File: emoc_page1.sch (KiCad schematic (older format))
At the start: 25 parts, among them U2 DRV8323R

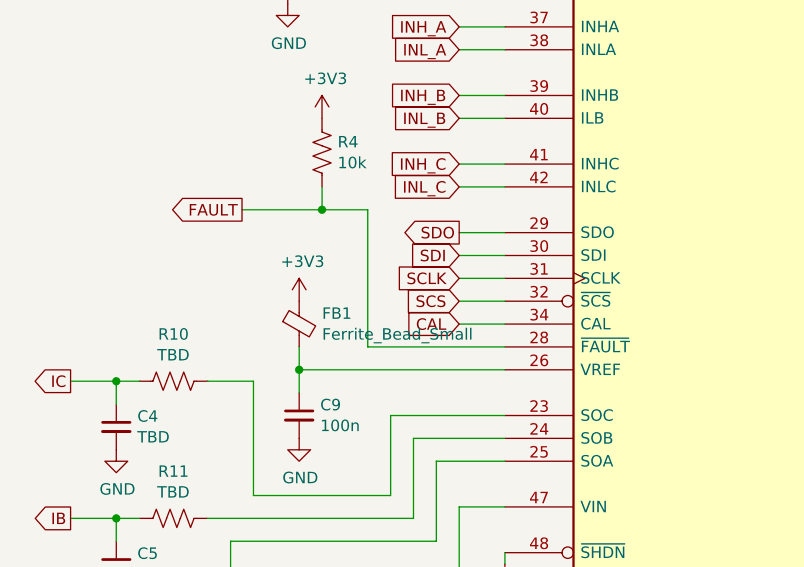
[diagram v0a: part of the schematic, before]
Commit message: still work in progress
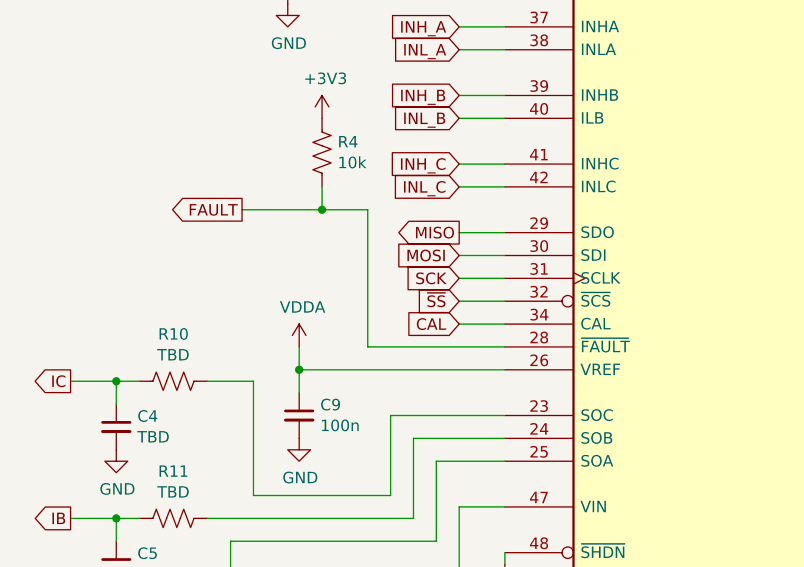
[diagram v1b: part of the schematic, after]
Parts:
- removed FB1: Ferrite_Bead_Small, symbol Device:Ferrite_Bead_Small
- C4, C5, C6, C9: footprint (none) -> Capacitor_SMD:C_0603_1608Metric
- NT1: footprint (none) -> NetTie:NetTie-2_SMD_Pad0.5mm
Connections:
- net VDDA: now reaches C9.1, U2.26 (VREF)
- net SCLK renamed SCK
- net SCS renamed ~SS
- net SDI renamed MOSI
- net SDO renamed MISO
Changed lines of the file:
@@
 $Descr A4 11693 8268
 encoding utf-8
-Sheet 2 4
+Sheet 2 5
 Title ""
 Date ""
@@
 F 0 "NT1" H 5950 1731 50  0000 C CNN
 F 1 "Net-Tie_2" H 5950 1640 50  0000 C CNN
-F 2 "" H 5950 1550 50  0001 C CNN
+F 2 "NetTie:NetTie-2_SMD_Pad0.5mm" H 5950 1550 50  0001 C CNN
 F 3 "~" H 5950 1550 50  0001 C CNN
 	1    5950 1550
@@
 $EndComp
 Text GLabel 3250 3650 0    50   Output ~ 0
-SDO
+MISO
 Text GLabel 3250 3750 0    50   Input ~ 0
-SDI
+MOSI
 Text GLabel 3250 3850 0    50   Input ~ 0
-SCLK
+SCK
 Text GLabel 3250 3950 0    50   Input ~ 0
-SCS
+~SS
 Wire Wire Line
 	3250 3750 3450 3750
@@
 F 0 "C9" H 2642 4496 50  0000 L CNN
 F 1 "100n" H 2642 4405 50  0000 L CNN
-F 2 "" H 2550 4450 50  0001 C CNN
+F 2 "Capacitor_SMD:C_0603_1608Metric" H 2550 4450 50  0001 C CNN
 F 3 "~" H 2550 4450 50  0001 C CNN
 	1    2550 4450
@@
 	2550 4250 2550 4150
 Connection ~ 2550 4250
-$Comp
-L power:+3V3 #PWR0110
-U 1 1 5FF033F4
-P 2550 3950
-F 0 "#PWR0110" H 2550 3800 50  0001 C CNN
-F 1 "+3V3" H 2565 4123 50  0000 C CNN
-F 2 "" H 2550 3950 50  0001 C CNN
-F 3 "" H 2550 3950 50  0001 C CNN
-	1    2550 3950
-	1    0    0    -1
-$EndComp
-$Comp
-L Device:Ferrite_Bead_Small FB1
-U 1 1 5FF0A0D9
-P 2550 4050
-F 0 "FB1" H 2650 4096 50  0000 L CNN
-F 1 "Ferrite_Bead_Small" H 2650 4005 50  0000 L CNN
-F 2 "" V 2480 4050 50  0001 C CNN
-F 3 "~" H 2550 4050 50  0001 C CNN
-	1    2550 4050
-	1    0    0    -1
-$EndComp
 Text GLabel 1550 5450 0    50   Output ~ 0
 IA
@@
 F 0 "C6" H 1842 5696 50  0000 L CNN
 F 1 "TBD" H 1842 5605 50  0000 L CNN
-F 2 "" H 1750 5650 50  0001 C CNN
+F 2 "Capacitor_SMD:C_0603_1608Metric" H 1750 5650 50  0001 C CNN
 F 3 "~" H 1750 5650 50  0001 C CNN
 	1    1750 5650
@@
 F 0 "C5" H 1842 5146 50  0000 L CNN
 F 1 "TBD" H 1842 5055 50  0000 L CNN
-F 2 "" H 1750 5100 50  0001 C CNN
+F 2 "Capacitor_SMD:C_0603_1608Metric" H 1750 5100 50  0001 C CNN
 F 3 "~" H 1750 5100 50  0001 C CNN
 	1    1750 5100
@@
 F 0 "C4" H 1842 4546 50  0000 L CNN
 F 1 "TBD" H 1842 4455 50  0000 L CNN
-F 2 "" H 1750 4500 50  0001 C CNN
+F 2 "Capacitor_SMD:C_0603_1608Metric" H 1750 4500 50  0001 C CNN
 F 3 "~" H 1750 4500 50  0001 C CNN
 	1    1750 4500
@@
 Wire Wire Line
 	7200 4200 7200 4300
+$Comp
+L power:VDDA #PWR08
+U 1 1 5FF1727A
+P 2550 4150
+F 0 "#PWR08" H 2550 4000 50  0001 C CNN
+F 1 "VDDA" H 2565 4323 50  0000 C CNN
+F 2 "" H 2550 4150 50  0001 C CNN
+F 3 "" H 2550 4150 50  0001 C CNN
+	1    2550 4150
+	1    0    0    -1
+$EndComp
 $EndSCHEMATC

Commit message: idk
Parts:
- C14: footprint (none) -> Capacitor_SMD:C_0603_1608Metric
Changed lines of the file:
@@
 F 0 "C14" H 6042 4246 50  0000 L CNN
 F 1 "100n" H 6042 4155 50  0000 L CNN
-F 2 "" H 5950 4200 50  0001 C CNN
+F 2 "Capacitor_SMD:C_0603_1608Metric" H 5950 4200 50  0001 C CNN
 F 3 "~" H 5950 4200 50  0001 C CNN
 	1    5950 4200
